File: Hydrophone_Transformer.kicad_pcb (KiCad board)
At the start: 2 copper layers, 14 x 30 mm, 1 part

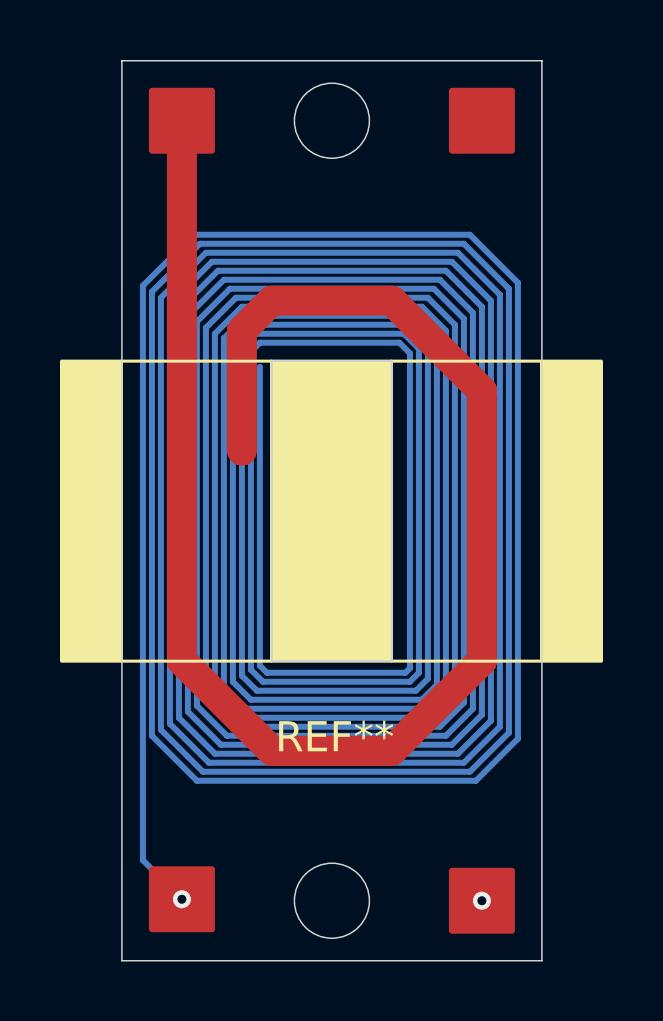
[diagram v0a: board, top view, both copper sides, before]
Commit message: poprawki Tadeusz
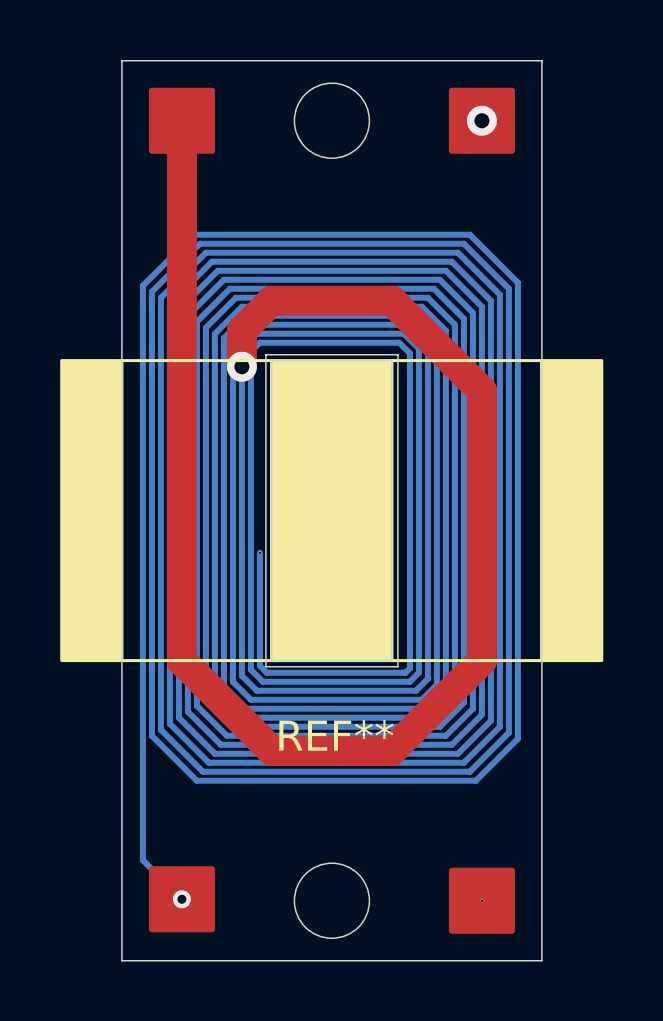
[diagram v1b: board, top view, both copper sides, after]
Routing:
- net GND: track 650.0 -> 645.2 mm, vias 2 -> 5
- added copper zone on In1.Cu, net GND
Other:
- outline, holes or cut-outs redrawn
- copper layers 2 -> 4
